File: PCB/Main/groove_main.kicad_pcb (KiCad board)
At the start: 2 copper layers, 214 x 99 mm, 50 parts, among them J1 Left_X, J10 Left_Y, J11 Right_X, J12 Right_Y, J2 Left_Y, J3 Right_X, J4 Right_Y, J5 Left_X, J6 Left_Y, J7 Right_X, J8 Right_Y, J9 Left_X, SW1 SWITCH_SPST, SW2 SWITCH_SPST, SW3 SWITCH_SPST, U1 Pico, U2 CD4052B, U3 LM4040DBZ-3

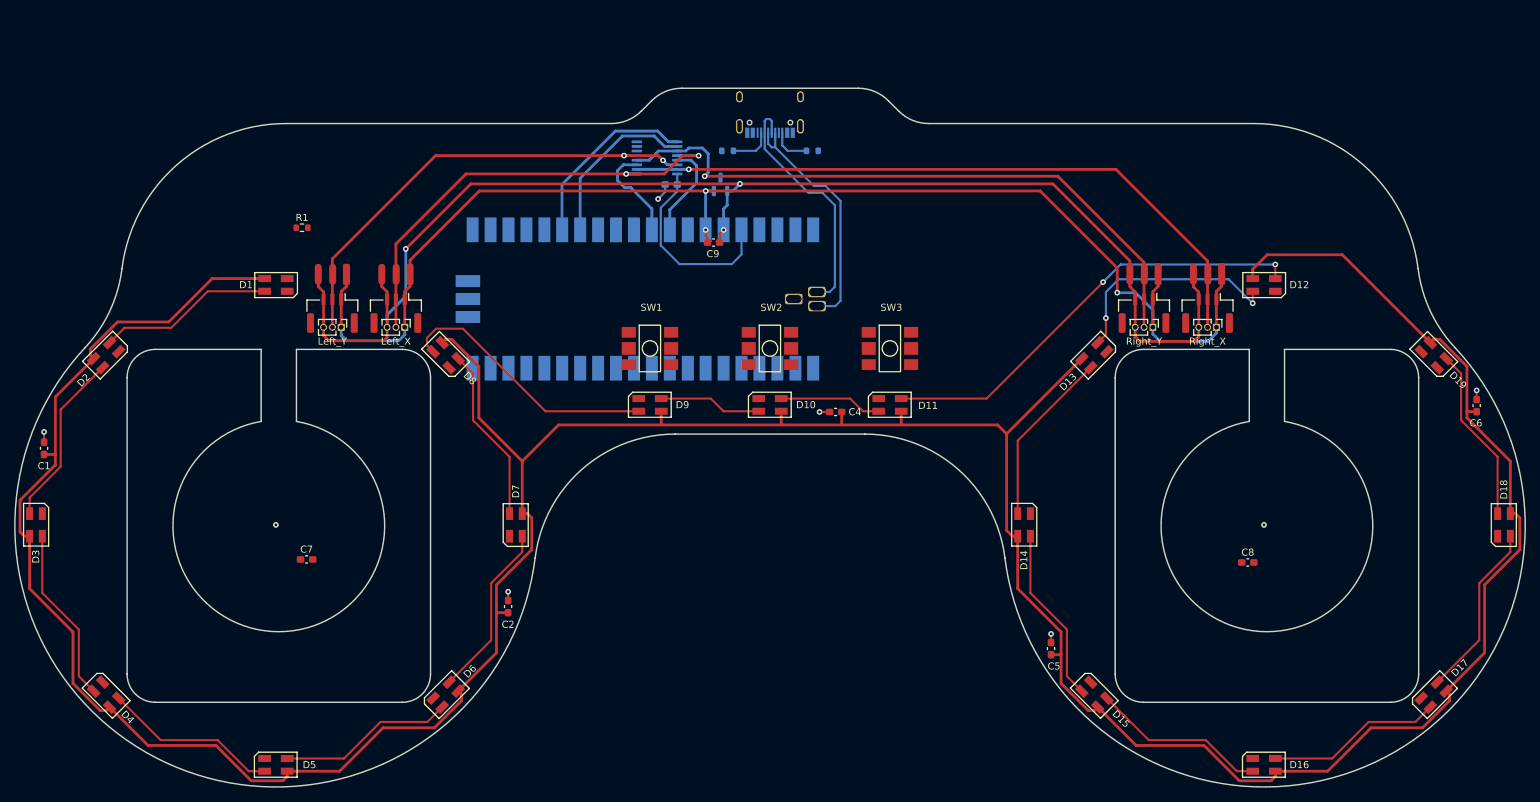
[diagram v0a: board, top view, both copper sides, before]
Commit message: Main PCB progress 70%
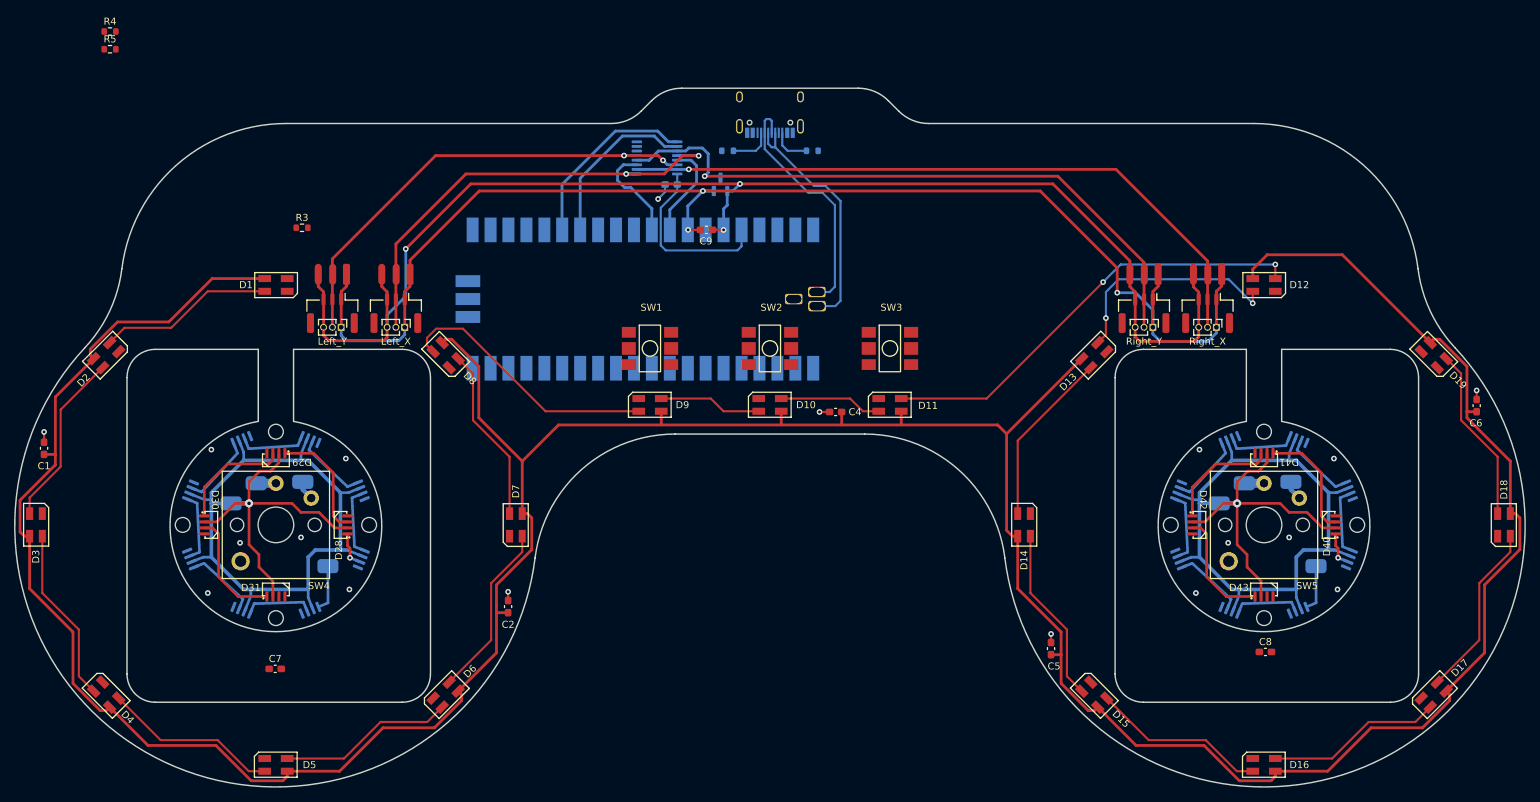
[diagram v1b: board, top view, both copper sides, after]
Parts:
- added D20: WS2812B_Unified, groove_pico:WS2812B-4020, B.Cu at (70.4, 126.1)
- added D21: WS2812B_Unified, groove_pico:WS2812B-4020, B.Cu at (60.2, 126.1)
- added D22: WS2812B_Unified, groove_pico:WS2812B-4020, B.Cu at (52.6, 118.5)
- added D23: WS2812B_Unified, groove_pico:WS2812B-4020, B.Cu at (52.6, 108.3)
- added D24: WS2812B_Unified, groove_pico:WS2812B-4020, B.Cu at (60.2, 100.7)
- added D25: WS2812B_Unified, groove_pico:WS2812B-4020, B.Cu at (70.4, 100.7)
- added D26: WS2812B_Unified, groove_pico:WS2812B-4020, B.Cu at (78.0, 108.3)
- added D27: WS2812B_Unified, groove_pico:WS2812B-4020, B.Cu at (78.0, 118.5)
- added D28: WS2812B_Unified, groove_pico:WS2812B-4020_UP, F.Cu at (76.1, 113.4)
- added D29: WS2812B_Unified, groove_pico:WS2812B-4020_UP, F.Cu at (65.3, 102.6)
- added D30: WS2812B_Unified, groove_pico:WS2812B-4020_UP, F.Cu at (54.5, 113.4)
- added D31: WS2812B_Unified, groove_pico:WS2812B-4020_UP, F.Cu at (65.3, 124.2)
- added D32: WS2812B_Unified, groove_pico:WS2812B-4020, B.Cu at (210.4, 126.1)
- added D33: WS2812B_Unified, groove_pico:WS2812B-4020, B.Cu at (200.2, 126.1)
- added D34: WS2812B_Unified, groove_pico:WS2812B-4020, B.Cu at (192.6, 118.5)
- added D35: WS2812B_Unified, groove_pico:WS2812B-4020, B.Cu at (192.6, 108.3)
- added D36: WS2812B_Unified, groove_pico:WS2812B-4020, B.Cu at (200.2, 100.7)
- added D37: WS2812B_Unified, groove_pico:WS2812B-4020, B.Cu at (210.4, 100.7)
- added D38: WS2812B_Unified, groove_pico:WS2812B-4020, B.Cu at (218.0, 108.3)
- added D39: WS2812B_Unified, groove_pico:WS2812B-4020, B.Cu at (218.0, 118.5)
- added D40: WS2812B_Unified, groove_pico:WS2812B-4020_UP, F.Cu at (216.1, 113.4)
- added D41: WS2812B_Unified, groove_pico:WS2812B-4020_UP, F.Cu at (205.3, 102.6)
- added D42: WS2812B_Unified, groove_pico:WS2812B-4020_UP, F.Cu at (194.5, 113.4)
- added D43: WS2812B_Unified, groove_pico:WS2812B-4020_UP, F.Cu at (205.3, 124.2)
- added J13: SW, groove_pico:Solder_1P, B.Cu at (69.1, 107.3)
- added J14: SW, groove_pico:Solder_1P, B.Cu at (209.1, 107.3)
- added J15: V, groove_pico:Solder_1P, B.Cu at (59.0, 110.4)
- added J16: LED, groove_pico:Solder_1P, B.Cu at (72.7, 119.2)
- added J18: G, groove_pico:Solder_1P, B.Cu at (62.5, 107.5)
- added J19: V, groove_pico:Solder_1P, B.Cu at (199.0, 110.4)
- added J20: LED, groove_pico:Solder_1P, B.Cu at (212.7, 119.2)
- added J22: G, groove_pico:Solder_1P, B.Cu at (202.5, 107.5)
- added R4: 10, Resistor_SMD:R_0603_1608Metric, F.Cu at (41.8, 43.5)
- added R5: 10, Resistor_SMD:R_0603_1608Metric, F.Cu at (41.8, 46.0)
- added SCR1: ScrewHole, groove_pico:Hole2.0, F.Cu at (65.3, 100.2)
- added SCR2: ScrewHole, groove_pico:Hole2.0, F.Cu at (78.5, 113.4)
- added SCR3: ScrewHole, groove_pico:Hole2.0, F.Cu at (65.3, 126.6)
- added SCR4: ScrewHole, groove_pico:Hole2.0, F.Cu at (52.1, 113.4)
- added SCR5: ScrewHole, groove_pico:Hole2.0, F.Cu at (205.3, 100.2)
- added SCR6: ScrewHole, groove_pico:Hole2.0, F.Cu at (218.5, 113.4)
- added SCR7: ScrewHole, groove_pico:Hole2.0, F.Cu at (205.3, 126.6)
- added SCR8: ScrewHole, groove_pico:Hole2.0, F.Cu at (192.1, 113.4)
- added SW4: SWITCH_SPST, groove_pico:SW_Kailh_Choc_V1V2_1.00u_LED, F.Cu at (65.3, 113.4)
- added SW5: SWITCH_SPST, groove_pico:SW_Kailh_Choc_V1V2_1.00u_LED, F.Cu at (205.3, 113.4)
- moved C7 16.1 mm to (65.2, 133.8)
- moved C8 12.9 mm to (205.5, 131.4)
- moved C9 2.06 mm to (126.3, 71.6)
- renumbered R2 to R1, R3 to R2, R1 to R3
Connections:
- SW1 pad 1: unconnected-(SW1-"~{"}-Pad1) -> Net-(U1-GPIO0)
- SW1 pad 2: unconnected-(SW1-"~{"}-Pad2) -> GND
- SW2 pad 1: unconnected-(SW2-"~{"}-Pad1) -> Net-(U1-GPIO1)
- SW2 pad 2: unconnected-(SW2-"~{"}-Pad2) -> GND
- SW3 pad 1: unconnected-(SW3-"~{"}-Pad1) -> Net-(U1-GPIO2)
- SW3 pad 2: unconnected-(SW3-"~{"}-Pad2) -> GND
- U1 pad 1: unconnected-(U1-GPIO0-Pad1) -> Net-(U1-GPIO0)
- U1 pad 13: unconnected-(U1-GND-Pad13) -> GND
- U1 pad 15: unconnected-(U1-GPIO11-Pad15) -> Net-(U1-GPIO11)
- U1 pad 16: /RGB -> Net-(U1-GPIO12)
- U1 pad 17: unconnected-(U1-GPIO13-Pad17) -> /RGB
- U1 pad 2: unconnected-(U1-GPIO1-Pad2) -> Net-(U1-GPIO1)
- U1 pad 23: unconnected-(U1-GND-Pad23) -> GND
- U1 pad 33: unconnected-(U1-AGND-Pad33) -> GNDREF
- U1 pad 34: GNDREF -> unconnected-(U1-GPIO28_ADC2-Pad34)
- U1 pad 4: unconnected-(U1-GPIO2-Pad4) -> Net-(U1-GPIO2)
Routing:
- net +5V: track 513.2 -> 796.8 mm, vias 0 -> 2
- net Net-(D30-Out): track 0.00 -> 16.5 mm
- net Net-(D40-Out): track 0.00 -> 16.5 mm
- net Net-(D28-Out): track 0.00 -> 16.5 mm
- net Net-(D42-Out): track 0.00 -> 16.5 mm
- net Net-(D41-Out): track 0.00 -> 16.3 mm
- net Net-(D29-Out): track 0.00 -> 16.3 mm
- net GND: track 9.07 -> 20.2 mm, vias 6 -> 18
- net Net-(D23-Out): track 0.00 -> 10.6 mm
- net Net-(D35-Out): track 0.00 -> 10.6 mm
- net Net-(D33-Out): track 0.00 -> 10.6 mm
- net Net-(D21-Out): track 0.00 -> 10.6 mm
- net Net-(D37-Out): track 0.00 -> 10.6 mm
- net Net-(D25-Out): track 0.00 -> 10.6 mm
- net Net-(D38-Out): track 0.00 -> 10.1 mm
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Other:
- outline, holes or cut-outs redrawn
